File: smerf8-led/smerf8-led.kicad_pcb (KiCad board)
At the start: 2 copper layers, 69 parts, among them J1 Conn_Coaxial_Small, J2 Conn_Coaxial_Small, J3 Conn_Coaxial_Small, J4 Conn_Coaxial_Small, U1 ERF8-ERM8-040-DV

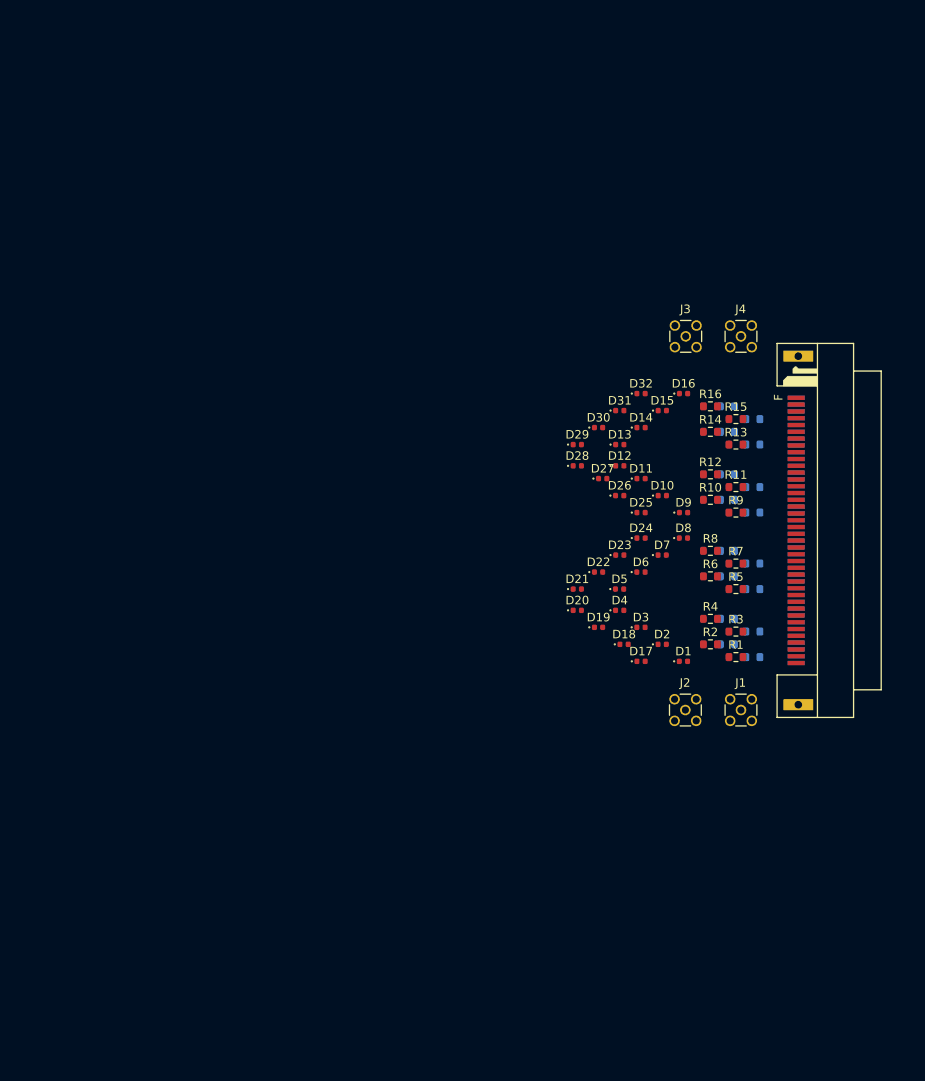
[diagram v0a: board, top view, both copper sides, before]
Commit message: board 90% done
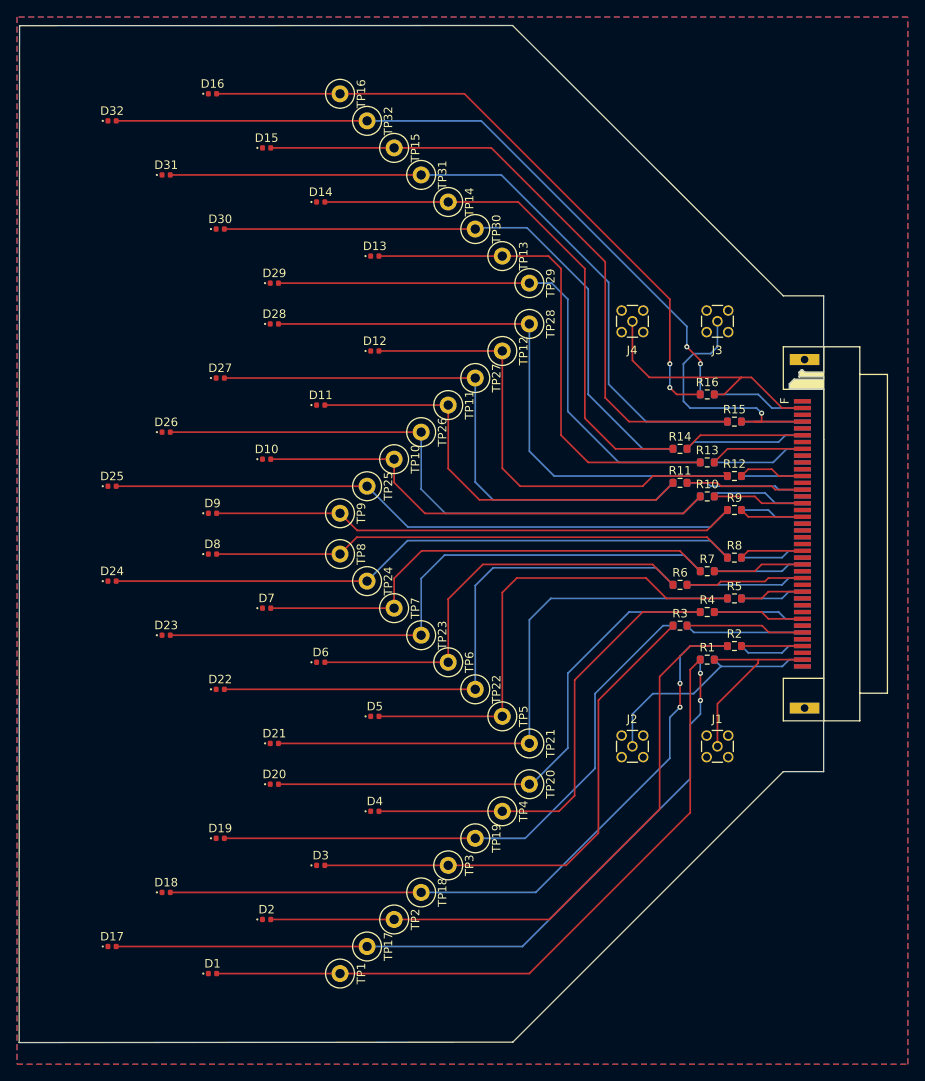
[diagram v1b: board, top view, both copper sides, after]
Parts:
- added TP1: TestPoint, cody:TestPoint_Plated_Hole_D1.1mm, F.Cu at (105.6, 136.7)
- added TP10: TestPoint, cody:TestPoint_Plated_Hole_D1.1mm, F.Cu at (112.0, 76.2)
- added TP11: TestPoint, cody:TestPoint_Plated_Hole_D1.1mm, F.Cu at (118.3, 69.9)
- added TP12: TestPoint, cody:TestPoint_Plated_Hole_D1.1mm, F.Cu at (124.7, 63.5)
- added TP13: TestPoint, cody:TestPoint_Plated_Hole_D1.1mm, F.Cu at (124.7, 52.3)
- added TP14: TestPoint, cody:TestPoint_Plated_Hole_D1.1mm, F.Cu at (118.3, 46.0)
- added TP15: TestPoint, cody:TestPoint_Plated_Hole_D1.1mm, F.Cu at (112.0, 39.6)
- added TP16: TestPoint, cody:TestPoint_Plated_Hole_D1.1mm, F.Cu at (105.6, 33.2)
- added TP17: TestPoint, cody:TestPoint_Plated_Hole_D1.1mm, F.Cu at (108.8, 133.5)
- added TP18: TestPoint, cody:TestPoint_Plated_Hole_D1.1mm, F.Cu at (115.1, 127.2)
- added TP19: TestPoint, cody:TestPoint_Plated_Hole_D1.1mm, F.Cu at (121.5, 120.8)
- added TP2: TestPoint, cody:TestPoint_Plated_Hole_D1.1mm, F.Cu at (112.0, 130.4)
- added TP20: TestPoint, cody:TestPoint_Plated_Hole_D1.1mm, F.Cu at (127.9, 114.5)
- added TP21: TestPoint, cody:TestPoint_Plated_Hole_D1.1mm, F.Cu at (127.9, 109.7)
- added TP22: TestPoint, cody:TestPoint_Plated_Hole_D1.1mm, F.Cu at (121.5, 103.3)
- added TP23: TestPoint, cody:TestPoint_Plated_Hole_D1.1mm, F.Cu at (115.1, 96.9)
- added TP24: TestPoint, cody:TestPoint_Plated_Hole_D1.1mm, F.Cu at (108.8, 90.6)
- added TP25: TestPoint, cody:TestPoint_Plated_Hole_D1.1mm, F.Cu at (108.8, 79.4)
- added TP26: TestPoint, cody:TestPoint_Plated_Hole_D1.1mm, F.Cu at (115.1, 73.0)
- added TP27: TestPoint, cody:TestPoint_Plated_Hole_D1.1mm, F.Cu at (121.5, 66.7)
- added TP28: TestPoint, cody:TestPoint_Plated_Hole_D1.1mm, F.Cu at (127.9, 60.3)
- added TP29: TestPoint, cody:TestPoint_Plated_Hole_D1.1mm, F.Cu at (127.9, 55.5)
- added TP3: TestPoint, cody:TestPoint_Plated_Hole_D1.1mm, F.Cu at (118.3, 124.0)
- added TP30: TestPoint, cody:TestPoint_Plated_Hole_D1.1mm, F.Cu at (121.5, 49.1)
- added TP31: TestPoint, cody:TestPoint_Plated_Hole_D1.1mm, F.Cu at (115.1, 42.8)
- added TP32: TestPoint, cody:TestPoint_Plated_Hole_D1.1mm, F.Cu at (108.8, 36.4)
- added TP4: TestPoint, cody:TestPoint_Plated_Hole_D1.1mm, F.Cu at (124.7, 117.6)
- added TP5: TestPoint, cody:TestPoint_Plated_Hole_D1.1mm, F.Cu at (124.7, 106.5)
- added TP6: TestPoint, cody:TestPoint_Plated_Hole_D1.1mm, F.Cu at (118.3, 100.1)
- added TP7: TestPoint, cody:TestPoint_Plated_Hole_D1.1mm, F.Cu at (112.0, 93.7)
- added TP8: TestPoint, cody:TestPoint_Plated_Hole_D1.1mm, F.Cu at (105.6, 87.4)
- added TP9: TestPoint, cody:TestPoint_Plated_Hole_D1.1mm, F.Cu at (105.6, 82.6)
- U1: footprint cody:ERF8-040-EM2 -> Library:ERF8-040-EM2
- moved D17 70.7 mm to (78.8, 133.5)
- moved D32 70.0 mm to (78.8, 36.4)
- moved D1 66.5 mm to (90.6, 136.7)
- moved D16 65.7 mm to (90.6, 33.2)
- moved D24 62.4 mm to (78.8, 90.6)
- moved D25 62.3 mm to (78.8, 79.4)
- moved D18 61.3 mm to (85.1, 127.2)
- moved D31 60.1 mm to (85.1, 42.8)
- moved D2 56.7 mm to (97.0, 130.4)
- moved D15 55.9 mm to (97.0, 39.6)
- moved D8 55.4 mm to (90.6, 87.4)
- moved D9 55.4 mm to (90.6, 82.6)
- moved D23 54.2 mm to (85.1, 96.9)
- moved D26 53.9 mm to (85.1, 73.0)
- moved D19 51.0 mm to (91.5, 120.8)
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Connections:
- J2 pad 1: sig02 -> sig17
- J3 pad 1: sig03 -> sig15
- J4 pad 1: sig04 -> sig16
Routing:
- net Net-(D17-A): track 0.00 -> 90.2 mm, vias 0 -> 2
- net Net-(D32-A): track 0.00 -> 85.8 mm, vias 0 -> 2
- net Net-(D31-A): track 0.00 -> 84.6 mm
- net Net-(D18-A): track 0.00 -> 83.9 mm, vias 0 -> 2
- net Net-(D1-A): track 0.00 -> 82.0 mm
- net Net-(D16-A): track 0.00 -> 77.6 mm, vias 0 -> 2
- net Net-(D15-A): track 0.00 -> 76.4 mm
- net Net-(D2-A): track 0.00 -> 76.2 mm
- net Net-(D25-A): track 0.00 -> 74.7 mm
- net Net-(D24-A): track 0.00 -> 74.7 mm
- net Net-(D26-A): track 0.00 -> 71.1 mm
- net Net-(D23-A): track 0.00 -> 70.9 mm
- net Net-(D30-A): track 0.00 -> 70.9 mm
- net Net-(D28-A): track 0.00 -> 69.0 mm
- net Net-(D21-A): track 0.00 -> 68.4 mm
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- added copper zone on B.Cu, net GND
- added copper zone on F.Cu, net GND
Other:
- board outline added: 94.7 x 119.6 mm
